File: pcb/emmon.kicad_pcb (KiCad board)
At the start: 4 copper layers, 47.3 x 67.2 mm, 46 parts, among them J1 PROG_CONN, J2 ANT_CONN, J3 AC_CONN, Q1 PT11-21C, U1 DS3231MZ, U2 AT24CS32-SSHM, U3 Ai-Thinker-Ra-01, U4 ESP-12F, U5 LM393

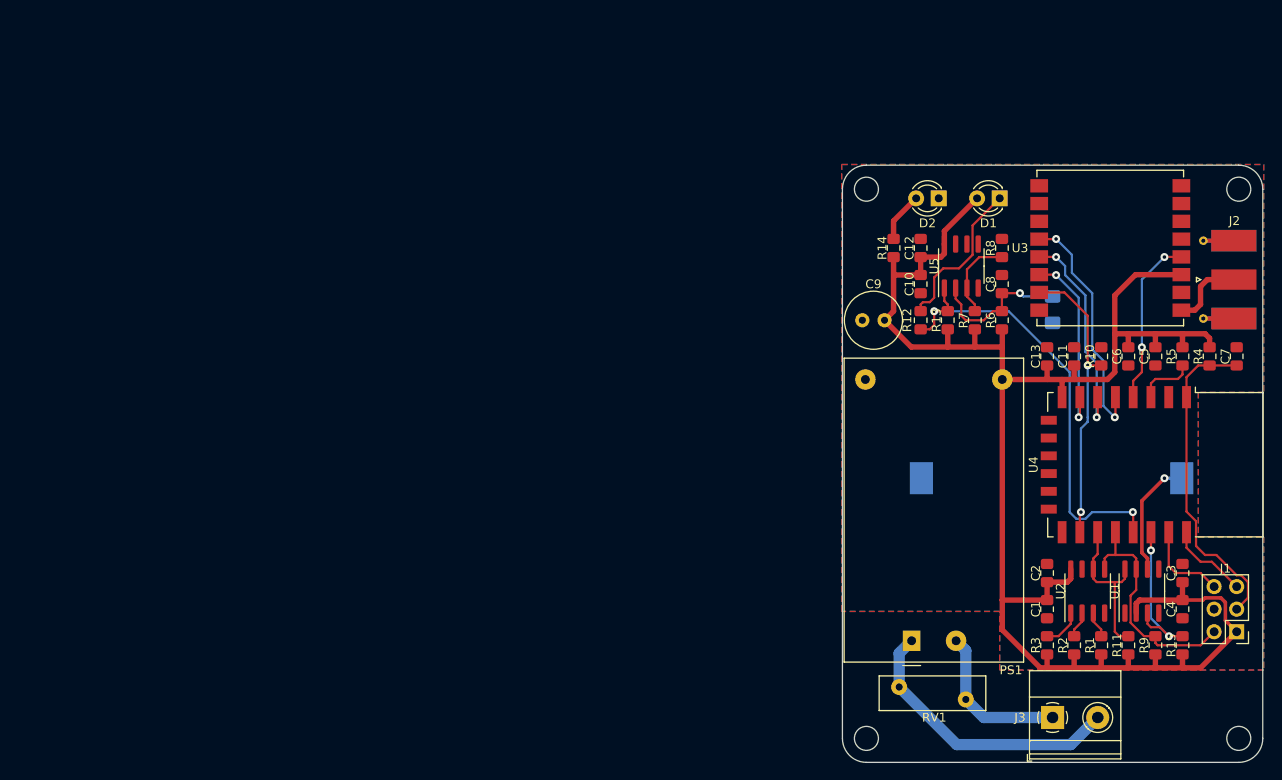
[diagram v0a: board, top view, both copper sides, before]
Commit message: Se corrigen las observaciones del docente
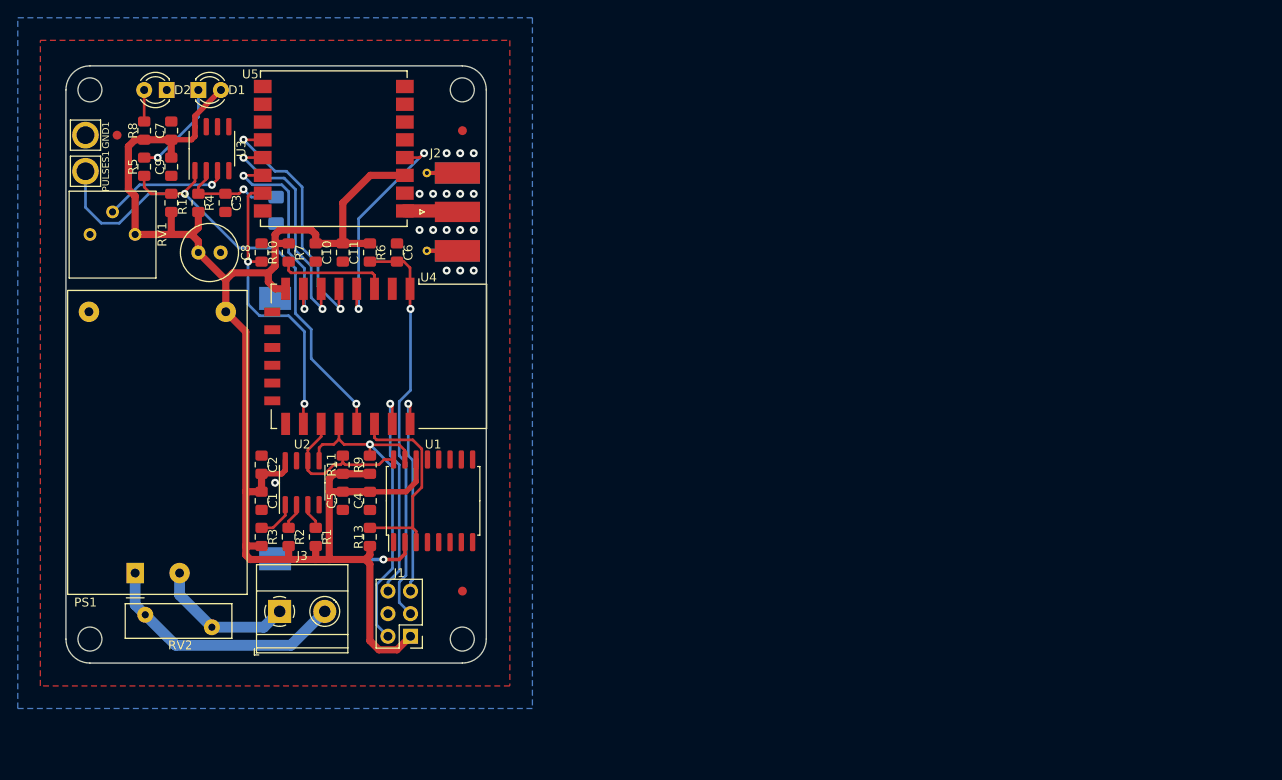
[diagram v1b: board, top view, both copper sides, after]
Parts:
- removed C12, C13: 100n, Capacitor_SMD:C_0805_2012Metric_Pad1.15x1.40mm_HandSolder
- removed R14, R15: 10K, Resistor_SMD:R_0805_2012Metric_Pad1.15x1.40mm_HandSolder
- added FID1: Fiducial, Fiducial:Fiducial_1mm_Mask2mm, F.Cu at (145.5, 122.4)
- added FID2: Fiducial, Fiducial:Fiducial_1mm_Mask2mm, F.Cu at (106.7, 71.1)
- added FID3: Fiducial, Fiducial:Fiducial_1mm_Mask2mm, F.Cu at (145.5, 70.6)
- added GND1: TestPoint, TestPoint:TestPoint_THTPad_3.0x3.0mm_Drill1.5mm, F.Cu at (103.1, 71.1)
- added PULSES1: TestPoint, TestPoint:TestPoint_THTPad_3.0x3.0mm_Drill1.5mm, F.Cu at (103.1, 75.2)
- added RV1: 10K, Potentiometer_THT:Potentiometer_Bourns_3386P_Vertical, F.Cu at (108.7, 82.3)
- BT1: value Battery -> BATTERY
- C11, C3, C5: value 1u -> 100n
- C4: value 100n -> 1u
- C6: value 100n -> 470p
- C7: value 470p -> 1u
- C8: value 100n -> 220u; footprint Capacitor_SMD:C_0805_2012Metric_Pad1.15x1.40mm_HandSolder -> Capacitor_THT:C_Radial_D6.3mm_H11.0mm_P2.50mm
- C9: value 220u -> 100n; footprint Capacitor_THT:C_Radial_D6.3mm_H11.0mm_P2.50mm -> Capacitor_SMD:C_0805_2012Metric_Pad1.15x1.40mm_HandSolder
- Q1: value PT11-21C -> PT11-21C/L41/TR8
- R12: value 1K -> 10K
- R5: value 10K -> 1K
- R7: value 5.1K -> 10K
- R8: value 5.1K -> 1K
- U1: value DS3231MZ -> DS3231SN; footprint Package_SO:SOIC-8_3.9x4.9mm_P1.27mm -> Package_SO:SOIC-16W_7.5x10.3mm_P1.27mm
- U2: value AT24CS32-SSHM -> CAT24C32WI-GT3
- U3: value Ai-Thinker-Ra-01 -> LM393DR2G; footprint RF_Module:Ai-Thinker-Ra-01-LoRa -> Package_SO:SOIC-8_3.9x4.9mm_P1.27mm
- U4: value ESP-12F -> ESP-12E
- U5: value LM393 -> Ai-Thinker-Ra-01; footprint Package_SO:SOIC-8_3.9x4.9mm_P1.27mm -> RF_Module:Ai-Thinker-Ra-01-LoRa
- moved C7 122.5 mm to (112.8, 70.6), turned to 90 degrees
- moved R5 118.8 mm to (109.7, 74.7), turned to 270 degrees
- moved C3 115.5 mm to (118.9, 78.7)
- moved R4 115.1 mm to (115.8, 78.7), turned to 270 degrees
- moved U3 101.7 mm to (117.3, 72.6), turned to 90 degrees
- moved R8 97.4 mm to (109.7, 70.6), turned to 90 degrees
- moved R10 95.2 mm to (122.9, 84.3), turned to 270 degrees
- moved J1 93.0 mm to (139.7, 127.5)
- moved C5 92.9 mm to (132.1, 112.3)
- moved C4 92.2 mm to (135.1, 112.3)
- moved D1 91.0 mm to (115.8, 66.0), turned to 0 degrees
- moved R9 90.7 mm to (135.1, 108.2), turned to 270 degrees
- moved R11 90.7 mm to (132.1, 108.2), turned to 270 degrees
- moved C8 90.5 mm to (115.8, 84.3), turned to 0 degrees
- moved R2 89.2 mm to (126.0, 116.3)
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- renumbered RV1 to RV2
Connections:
- net ACL renamed Net-(J3-Pad2)
- net ACN renamed Net-(J3-Pad1)
- net RXD renamed /RXD
- net TXD renamed /TXD
- C3 pad 1: +3V3 -> GND
- C3 pad 2: GND -> Net-(C3-Pad2)
- C6 pad 1: +3V3 -> GND
- C6 pad 2: GND -> /RST
- C7 pad 1: GND -> +3V3
- C7 pad 2: RST -> GND
- C8 pad 1: GND -> +3V3
- C8 pad 2: Net-(C8-Pad2) -> GND
- J1 pad 2: SDA -> /SDA
- J1 pad 3: RST -> /RST
- J2 pad 1: ANT -> Net-(J2-Pad1)
- Q1 pad 1: Net-(C8-Pad2) -> Net-(C3-Pad2)
- R10 pad 1: NSS -> GND
- R10 pad 2: GND -> Net-(R10-Pad2)
- R11 pad 1: +3V3 -> /SCL
- R11 pad 2: SCL -> +3V3
- R12 pad 1: Net-(D1-Pad1) -> /PULSES
- R12 pad 2: PULSES -> +3V3
- R13 pad 1: +3V3 -> /ALARM
- R13 pad 2: PULSES -> +3V3
- R4 pad 1: RST -> Net-(C3-Pad2)
- R5 pad 1: Net-(R5-Pad1) -> Net-(D1-Pad1)
- R5 pad 2: +3V3 -> /PULSES
- R6 pad 1: Net-(C8-Pad2) -> /RST
- R8 pad 1: GND -> +3V3
- R8 pad 2: Net-(R7-Pad1) -> Net-(D2-Pad2)
- R9 pad 1: +3V3 -> /SDA
- R9 pad 2: SDA -> +3V3
- U1 pad 2: +3V3 -> Net-(BT1-Pad1)
- U1 pad 3: ALARM -> /ALARM
- U1 pad 6: Net-(BT1-Pad1) -> GND
- U1 pad 7: SDA -> GND
- U1 pad 8: SCL -> GND
- U2 pad 5: SDA -> /SDA
- U2 pad 6: SCL -> /SCL
- U3 pad 1: ANT -> /PULSES
- U3 pad 2: GND -> Net-(C3-Pad2)
- U3 pad 3: +3V3 -> Net-(RV1-Pad2)
- U3 pad 4: RESET -> GND
- U3 pad 8: (no net) -> +3V3
- U4 pad 1: RST -> /RST
- U4 pad 16: NSS -> Net-(R10-Pad2)
- U4 pad 17: SCL -> /SCL
- U4 pad 18: SDA -> /SDA
- U4 pad 19: PULSES -> /PULSES
- U4 pad 20: ALARM -> /ALARM
- U4 pad 3: Net-(R5-Pad1) -> Net-(R7-Pad1)
- U4 pad 4: RESET -> Net-(U4-Pad4)
- U4 pad 5: SCK -> Net-(U4-Pad5)
- U4 pad 6: MISO -> Net-(U4-Pad6)
- U4 pad 7: MOSI -> Net-(U4-Pad7)
- U5 pad 1: PULSES -> Net-(J2-Pad1)
- U5 pad 2: Net-(C8-Pad2) -> GND
- U5 pad 3: Net-(R7-Pad1) -> +3V3
- U5 pad 4: GND -> Net-(U4-Pad4)
- U5 pad 8: +3V3 -> (no net)
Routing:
- net /PULSES: track 0.00 -> 62.9 mm, vias 0 -> 2
- net PULSES: track 51.4 -> 0.00 mm, vias 2 -> 0
- net /RST: track 0.00 -> 45.4 mm, vias 0 -> 1
- net /SDA: track 0.00 -> 39.9 mm, vias 0 -> 1
- net RST: track 36.7 -> 0.00 mm
- net Net-(R10-Pad2): track 0.00 -> 33.5 mm, vias 0 -> 2
- net NSS: track 32.8 -> 0.00 mm, vias 2 -> 0
- net Net-(U4-Pad5): track 0.00 -> 28.8 mm, vias 0 -> 2
- net SCK: track 27.0 -> 0.00 mm, vias 2 -> 0
- net SDA: track 26.7 -> 0.00 mm
- net Net-(U4-Pad6): track 0.00 -> 26.5 mm, vias 0 -> 2
- net Net-(U4-Pad4): track 0.00 -> 25.3 mm, vias 0 -> 2
- net Net-(U4-Pad7): track 0.00 -> 24.3 mm, vias 0 -> 2
- net MISO: track 24.1 -> 0.00 mm, vias 2 -> 0
- net /ALARM: track 0.00 -> 23.3 mm
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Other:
- copper layers 4 -> 2
- net class Default: clearance 0.127 -> 0.1778; trace_width 0.127 -> 0.3048; via_dia 0.6 -> 0.9; via_drill 0.3 -> 0.4
- rule trace_clearance: 0.127 -> 0.1778
- rule trace_min: 0.127 -> 0.254
- board text added: "Mínimos (JLCPCP - 2 capas): Grillas: 0,508 mm (posicionamiento), 0,254 mm (ruteo), 0,1 mm (borde PCB) Vía: 0,6 mm / 0,3 mm Márgen: 0,127 mm Pista: 0,127 mm Dist. a borde: 0.2 mm Terminación: HASL"
- board text added: "Notas: - El borde del PCB se realizó según las medidas de la caja VG-S43 de la marca Vange. - La ubicación de los componentes se realizó priorizando que los conector se encuentren en el borde de la placa y que U5 t J2 se ecuentren lo más cerca posible entre ellos. - La ubicación de Q1 está bloqueada para que coincida el agujero inferior de la caja"
